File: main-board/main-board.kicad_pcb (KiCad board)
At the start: 2 copper layers, 180 x 111 mm, 63 parts, among them J1 INPUT, J2 NC1, J3 OUTPUT, J4 Conn_01x03_Pin, J5 COM, J6 INPUT_DEBUG, J7 NC__DEBUG, J8 OUTPUT_DEBUG, SW1 SW_SPST, SW2 Power Switch A, SW3 Power Switch B, U1 ADA4898-2, U2 ADA4898-2, U3 AD633ANZ

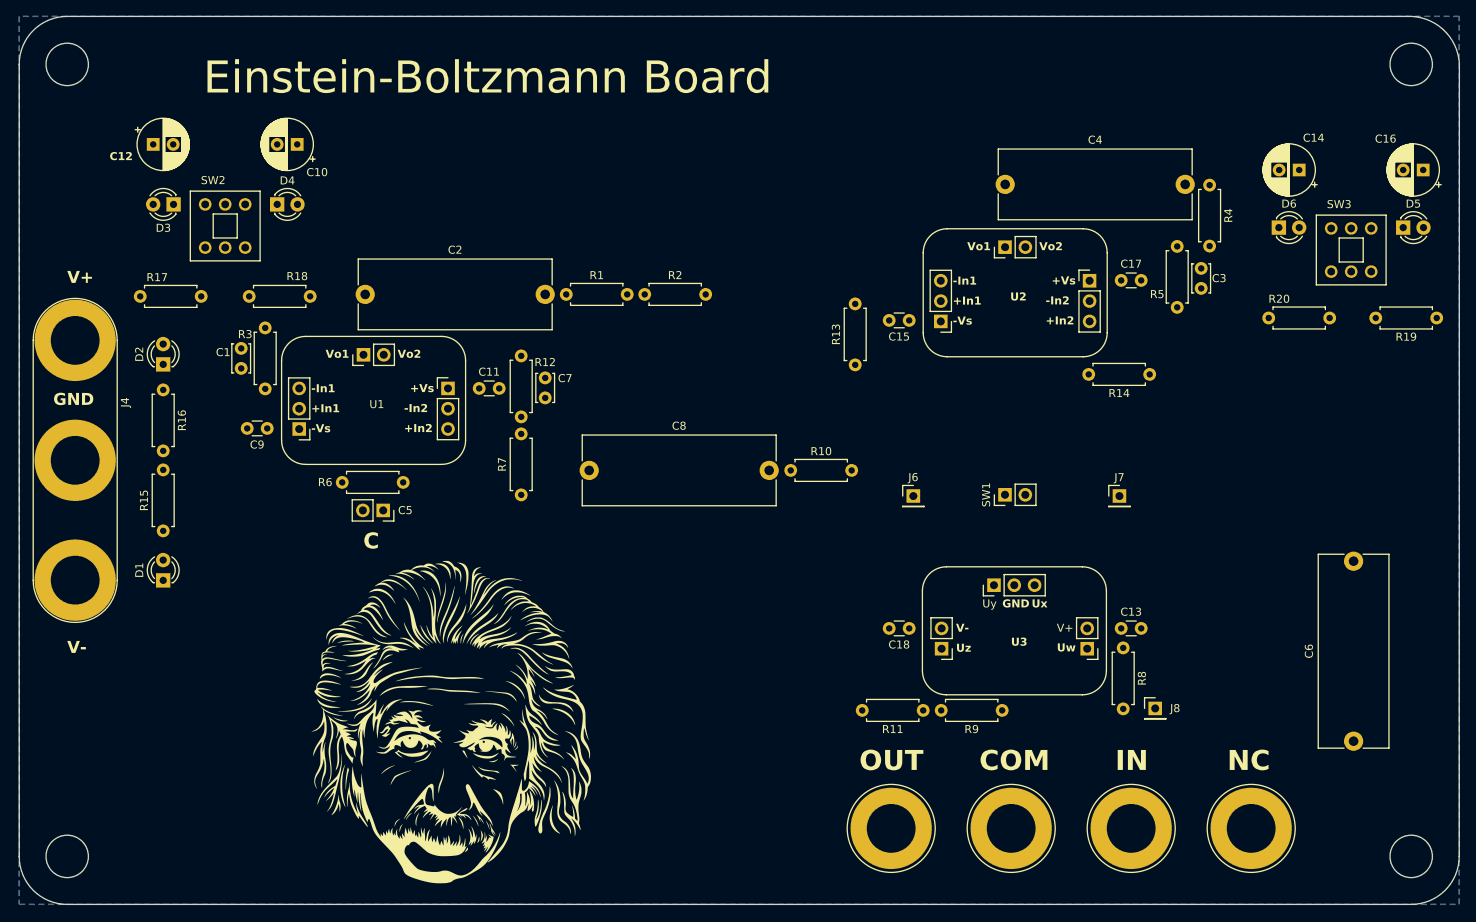
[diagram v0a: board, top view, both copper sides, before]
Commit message: Continues placement process
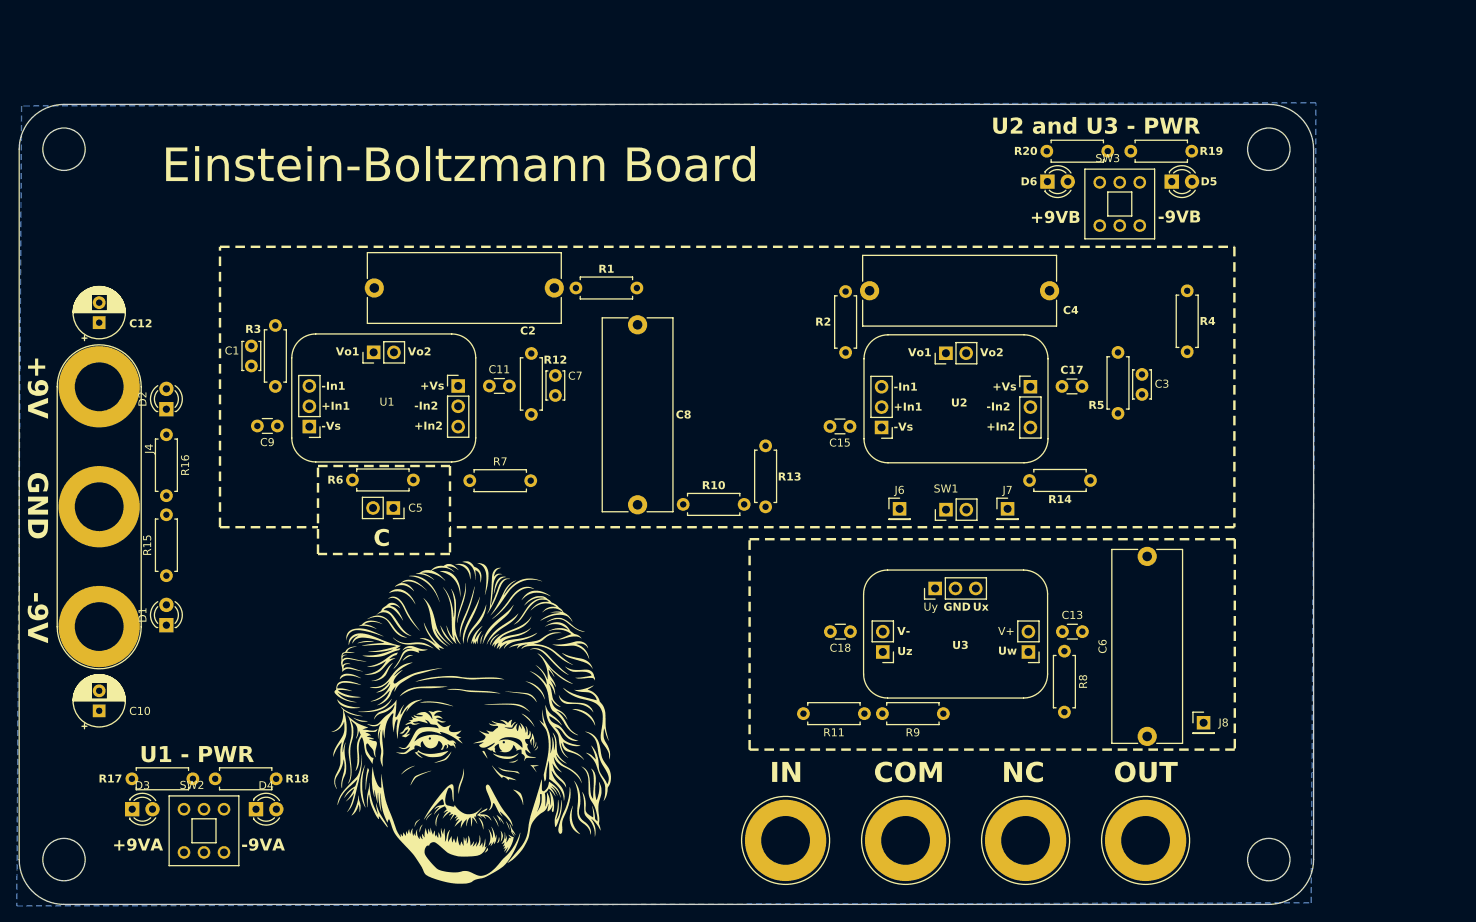
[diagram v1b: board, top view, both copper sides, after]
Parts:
- removed C14, C16: 10u, Capacitor_THT:CP_Radial_D6.3mm_P2.50mm
- moved D3 75.8 mm to (74.1, 142.1), turned to 0 degrees
- moved D4 75.6 mm to (89.6, 142.1)
- moved SW2 75.6 mm to (80.6, 142.1)
- moved C10 75.0 mm to (70.0, 129.8), turned to 90 degrees
- moved R18 60.4 mm to (92.1, 138.3)
- moved R17 60.3 mm to (74.1, 138.3)
- moved J1 43.2 mm to (155.8, 146.0)
- moved R19 37.0 mm to (206.6, 59.9)
- moved R20 34.7 mm to (188.4, 59.9)
- moved J3 31.8 mm to (200.8, 146.0)
- moved D5 29.5 mm to (204.1, 63.6)
- moved D6 29.5 mm to (188.5, 63.6)
- moved SW3 29.5 mm to (195.1, 63.8)
- moved J2 28.2 mm to (185.8, 146.0)
- moved R2 26.1 mm to (163.3, 85.0), turned to 90 degrees
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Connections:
- C10 pad 2: -9VA -> -9V
- C12 pad 1: +9VA -> +9V
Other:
- board size 180 x 111 mm -> 161.8 x 100 mm
- board text added: "+9V"
- board text added: "+9VA"
- board text added: "+9VB"
- board text added: "-9V"
- board text added: "-9VA"
- board text added: "-9VB"
- board text added: "U1 - PWR"
- board text added: "U2 and U3 - PWR"
- board text removed: "V+"
- board text removed: "V-"
